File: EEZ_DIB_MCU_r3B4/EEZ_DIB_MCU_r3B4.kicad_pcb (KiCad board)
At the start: 4 copper layers, 139.5 x 70 mm, 114 parts, among them IC1 TPD4E001DRLR, IC11 TPS2051BDBVR, IC12 TPS61169DCKR, IC13 TPD4E001DRLR, IC14 TSC2007IPW, IC2 74AUP1G74DC.125, IC3 CD74HC4050PWR, IC5 LD1117ADT33TR, IC8 AT24C256C-SSHL-B, IC9 N.C., J1 5033981892, J2 67803-8020, J3 HR911130A, Q1 N.C., Q2 2N7002, SW1 TL1100CF160Q, SW2 PEC16-2215F-S0024, U1 ICN6211, X1 DS1024-2*20R0, X2 DS1013-16SSIB1, X3 691322110005

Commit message: Adding connections to Ethernet connector
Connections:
- J3 pad 1: unconnected-(J3-P1-Pad1) -> Net-(J3-P1)
- J3 pad 10: unconnected-(J3-P10-Pad10) -> Net-(J3-P10)
- J3 pad 11: unconnected-(J3-Pad11) -> Net-(J3-Pad11)
- J3 pad 12: unconnected-(J3-Pad12) -> GND
- J3 pad 13: unconnected-(J3-Pad13) -> GND
- J3 pad 14: unconnected-(J3-Pad14) -> Net-(J3-Pad14)
- J3 pad 2: unconnected-(J3-P2-Pad2) -> /CM4_IO_slow/eth_0p
- J3 pad 3: unconnected-(J3-P3-Pad3) -> /CM4_IO_slow/eth_0n
- J3 pad 4: unconnected-(J3-P4-Pad4) -> /CM4_IO_slow/eth_1p
- J3 pad 5: unconnected-(J3-P5-Pad5) -> /CM4_IO_slow/eth_2p
- J3 pad 6: unconnected-(J3-P6-Pad6) -> /CM4_IO_slow/eth_2n
- J3 pad 7: unconnected-(J3-P7-Pad7) -> /CM4_IO_slow/eth_1n
- J3 pad 8: unconnected-(J3-P8-Pad8) -> /CM4_IO_slow/eth_3p
- J3 pad 9: unconnected-(J3-P9-Pad9) -> /CM4_IO_slow/eth_3n
- J3 pad S1: Net-(J3-SHIELD-PadS1) -> GND
- J3 pad S2: Net-(J3-SHIELD-PadS1) -> GND
- Module1 pad 10: unconnected-(Module1A-Ethernet_Pair0_N-Pad10) -> /CM4_IO_slow/eth_0n
- Module1 pad 11: unconnected-(Module1A-Ethernet_Pair2_P-Pad11) -> /CM4_IO_slow/eth_2n
- Module1 pad 12: unconnected-(Module1A-Ethernet_Pair0_P-Pad12) -> /CM4_IO_slow/eth_0p
- Module1 pad 15: unconnected-(Module1A-Ethernet_nLED3(3.3v)-Pad15) -> /CM4_IO_slow/eth_led3
- Module1 pad 17: unconnected-(Module1A-Ethernet_nLED2(3.3v)-Pad17) -> /CM4_IO_slow/eth_led2
- Module1 pad 19: unconnected-(Module1A-Ethernet_nLED1(3.3v)-Pad19) -> /CM4_IO_slow/eth_led1
- Module1 pad 3: unconnected-(Module1A-Ethernet_Pair3_P-Pad3) -> /CM4_IO_slow/eth_3p
- Module1 pad 4: unconnected-(Module1A-Ethernet_Pair1_P-Pad4) -> /CM4_IO_slow/eth_1p
- Module1 pad 5: unconnected-(Module1A-Ethernet_Pair3_N-Pad5) -> /CM4_IO_slow/eth_3n
- Module1 pad 6: unconnected-(Module1A-Ethernet_Pair1_N-Pad6) -> /CM4_IO_slow/eth_1n
- Module1 pad 9: unconnected-(Module1A-Ethernet_Pair2_N-Pad9) -> /CM4_IO_slow/eth_2p

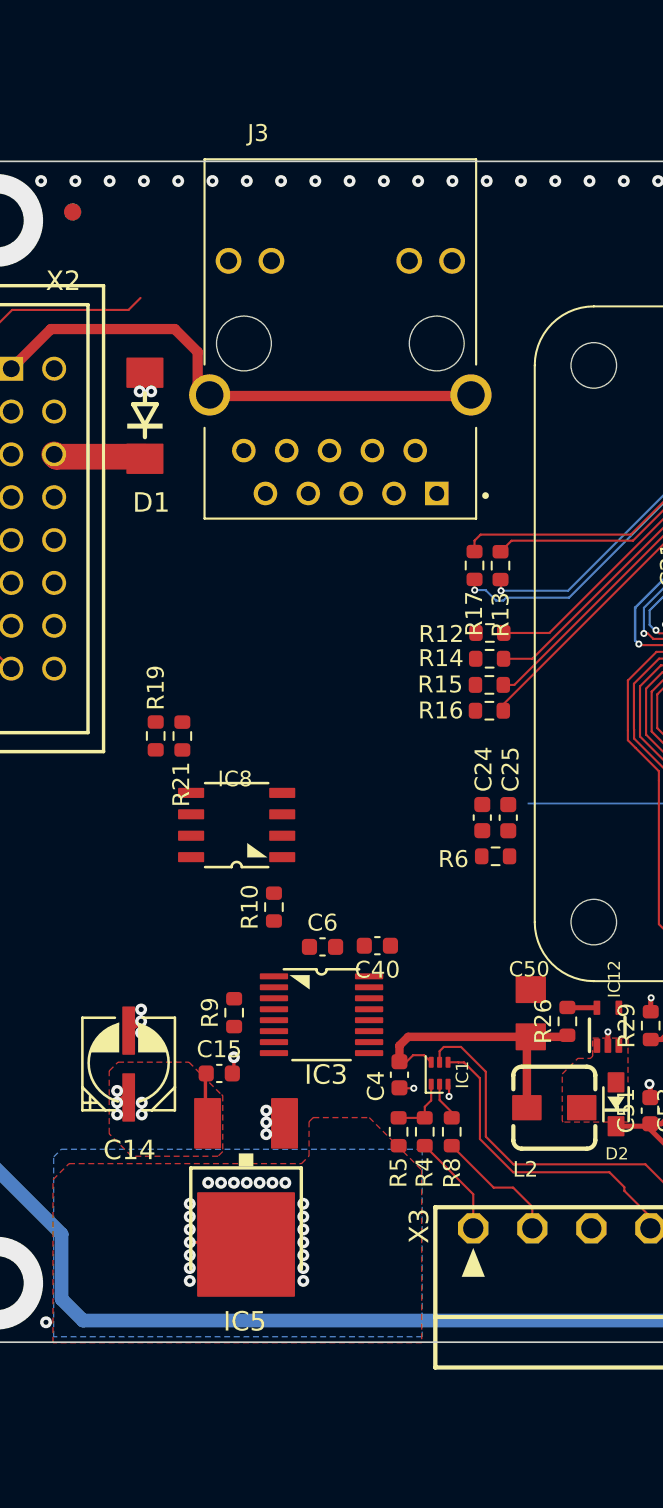
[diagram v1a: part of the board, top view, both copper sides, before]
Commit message: Adding DSI connector
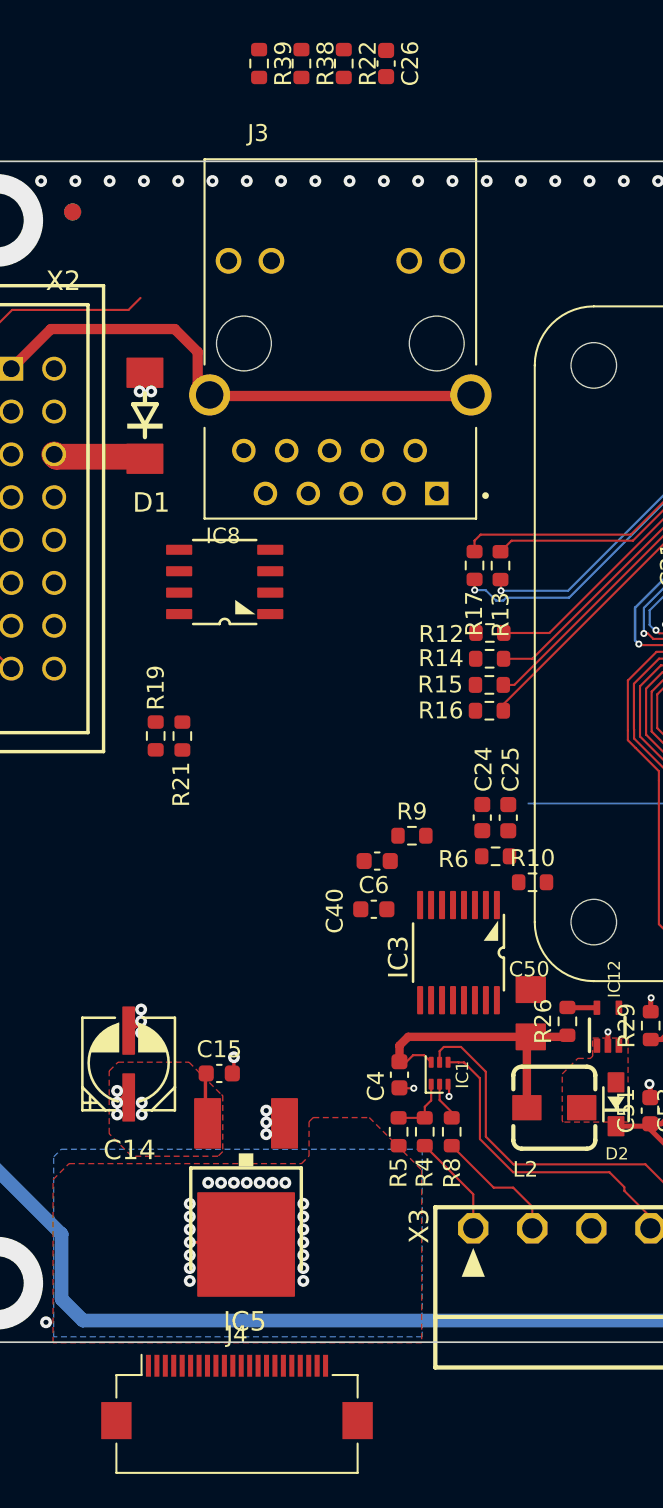
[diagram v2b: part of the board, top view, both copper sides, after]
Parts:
- added C26: C_Small, Capacitor_SMD:C_0603_1608Metric, F.Cu at (53.0, 56.8)
- added J4: Conn_01x22_Socket, Connector_FFC-FPC:Hirose_FH12-22S-0.5SH_1x22-1MP_P0.50mm_Horizontal, F.Cu at (44.1, 135.8)
- added R22: R_Small, Resistor_SMD:R_0603_1608Metric, F.Cu at (50.5, 56.8)
- added R38: R_Small, Resistor_SMD:R_0603_1608Metric, F.Cu at (48.0, 56.8)
- added R39: R_Small, Resistor_SMD:R_0603_1608Metric, F.Cu at (45.5, 56.8)
- moved R10 15.4 mm to (61.7, 105.3), turned to 0 degrees
- moved R9 14.9 mm to (54.5, 102.5), turned to 0 degrees
- moved IC8 14.4 mm to (43.4, 87.5)
- moved IC3 8.91 mm to (57.3, 109.5), turned to -90 degrees
- moved C40 5.02 mm to (52.5, 104.0)
- moved C6 3.77 mm to (52.3, 106.9)
